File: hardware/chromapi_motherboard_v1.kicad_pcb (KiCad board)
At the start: 4 copper layers, 105.4 x 57.9 mm, 139 parts, among them J1 Battery Input, J10 Top Left Switch, J11 Top Right Switch, J12 Bottom Left Switch, J13 Bottom Right Switch, J14 RPI_Connector, J2 Power Switch, J3 USB_C_Receptacle_USB2.0_14P, J4 Conn_ST_STDC14, J5 Conn_TopLeft, J6 Conn_TopRight, J7 Conn_BotLeft, J8 Conn_BotRight, J9 Speaker connector, M1 Noctua NF-A4x10, Q1 CSD17581Q3A, Q2 CSD17581Q3A, Q3 AO4435, Q4 AO4468, U1 HY2120, U10 MAX98357A, U11 BMI088, U2 INA226, U3 CN3302, U4 TPS51388VABR, U5 LD39050PU33R, U6 SN74LVC1G126DBVR, U7 STM32G431KBTx, U8 SN74LVC1G125DBVR, U9 SN74AHCT1G125DBVR

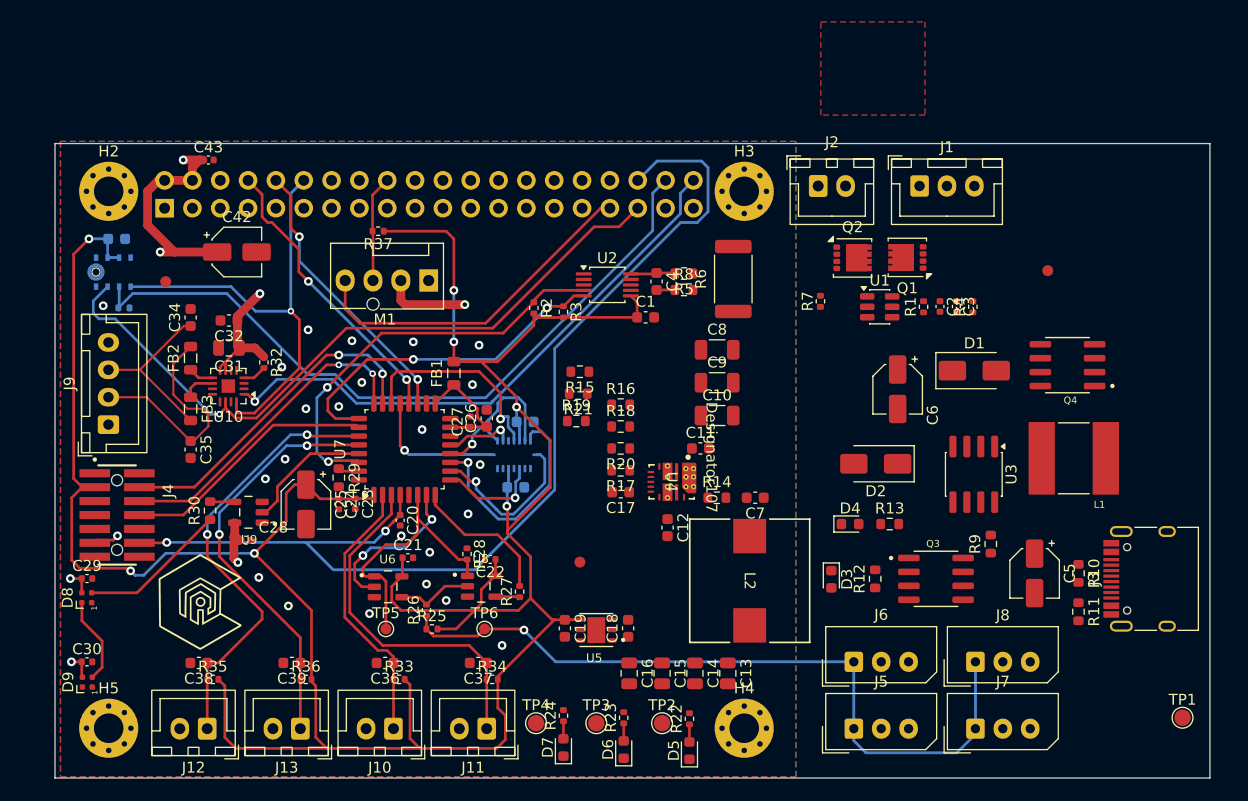
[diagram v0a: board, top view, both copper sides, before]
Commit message: Routing update
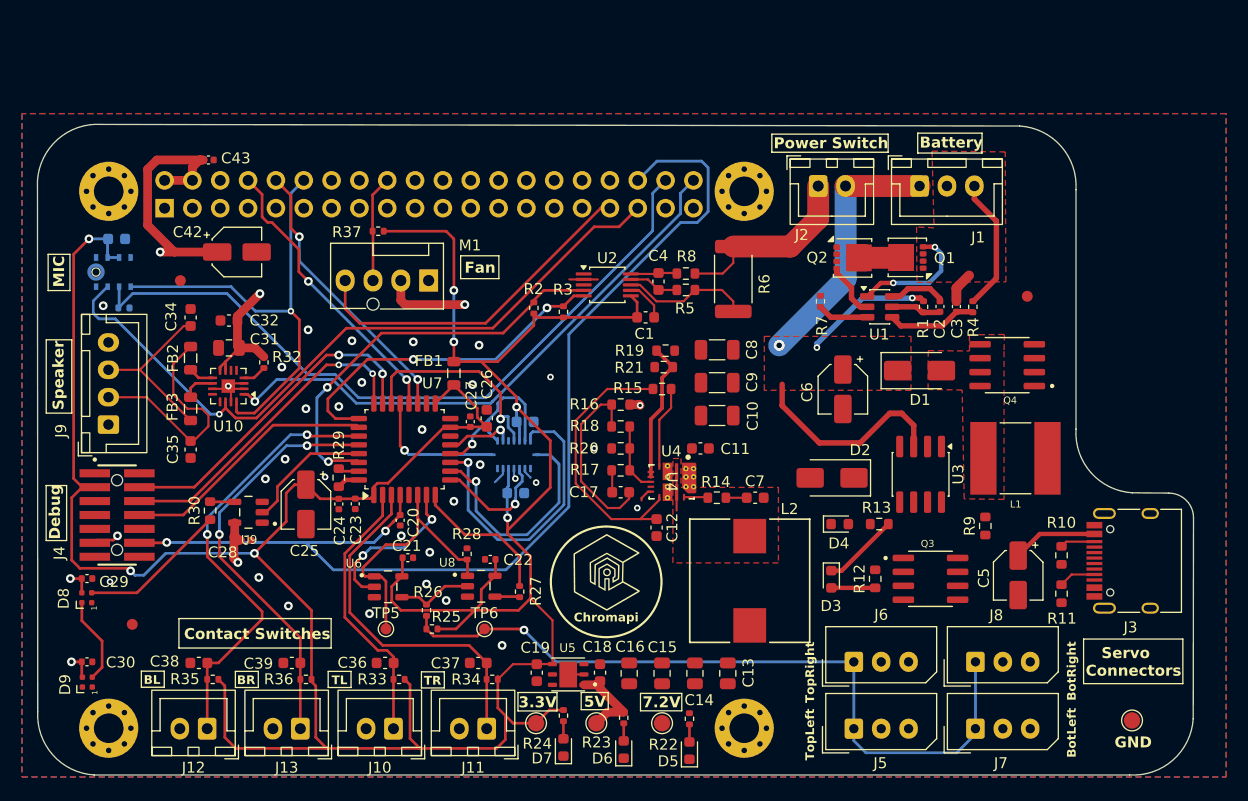
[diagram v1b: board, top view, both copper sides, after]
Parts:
- moved FID2 41.2 mm to (109.2, 113.0)
- moved H1 37.2 mm to (152.4, 108.3)
- moved R19 10.4 mm to (157.8, 88.0), turned to 180 degrees
- moved R21 8.17 mm to (157.7, 89.5)
- moved R15 7.66 mm to (157.5, 91.5)
- moved Q4 5.50 mm to (189.0, 89.3)
- moved L1 5.32 mm to (189.8, 97.8)
- moved C6 5.00 mm to (174.0, 91.5)
- moved D1 5.00 mm to (181.0, 89.8)
- moved U3 4.85 mm to (181.1, 99.3)
- moved C18 4.79 mm to (151.8, 117.4)
- moved C19 4.79 mm to (146.1, 117.4)
- moved U5 4.79 mm to (148.9, 117.5)
- moved TP1 4.62 mm to (200.4, 121.8)
- moved D2 4.18 mm to (173.0, 99.6)
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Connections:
- J1 pad 2: /Power Supply & Charge/BM -> /Power Supply & Charge/B-
- J1 pad 3: /Power Supply & Charge/B- -> /Power Supply & Charge/BM
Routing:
- net /Power Supply & Charge/B+: track 0.00 -> 55.8 mm, vias 0 -> 3
- net Net-(U4-VCC): track 0.00 -> 25.4 mm
- net GND: track 2.34 -> 22.9 mm, vias 24 -> 32
- net /Power Supply & Charge/V_BATT: track 0.00 -> 17.2 mm
- net Net-(C17-Pad1): track 0.00 -> 17.1 mm
- net +3.3V: track 263.1 -> 278.9 mm
- net +5V: track 49.2 -> 63.9 mm
- net /Voltage regulation/EN: track 0.00 -> 13.1 mm
- net /Power Supply & Charge/BM: track 0.00 -> 12.3 mm
- net /Power Supply & Charge/V_SYS: track 0.00 -> 11.8 mm
- net Net-(Q1-G): track 0.00 -> 11.2 mm, vias 0 -> 2
- net Net-(U1-VC): track 0.00 -> 8.25 mm
- net /Power Supply & Charge/B-: track 0.00 -> 8.10 mm
- net Net-(U3-CE): track 0.00 -> 7.77 mm
- net Net-(U4-PG): track 0.00 -> 7.52 mm
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- added copper zone on F.Cu, net /Power Supply & Charge/B-
- added copper zone on F.Cu, net Net-(C7-Pad1)
- added copper zone on F.Cu, net Net-(D1-A)
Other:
- board size 105.4 x 57.9 mm -> 105.5 x 59.4 mm
- board text added: "3.3V"
- board text added: "5V"
- board text added: "7.2V"
- board text added: "BL"
- board text added: "BR"
- board text added: "Battery"
- board text added: "BotLeft"
- board text added: "BotRight"
- board text added: "Chromapi"
- board text added: "Contact Switches"
- board text added: "Debug"
- board text added: "Fan"
- board text added: "GND"
- board text added: "IMU"
- board text added: "MIC"
- board text added: "Power Switch"
- board text added: "Servo Connectors"
- board text added: "Speaker"
- board text added: "TL"
- board text added: "TR"
- board text added: "TopLeft"
- board text added: "TopRight"
